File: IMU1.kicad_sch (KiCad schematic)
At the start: 3 parts, among them U2 262-BMI088

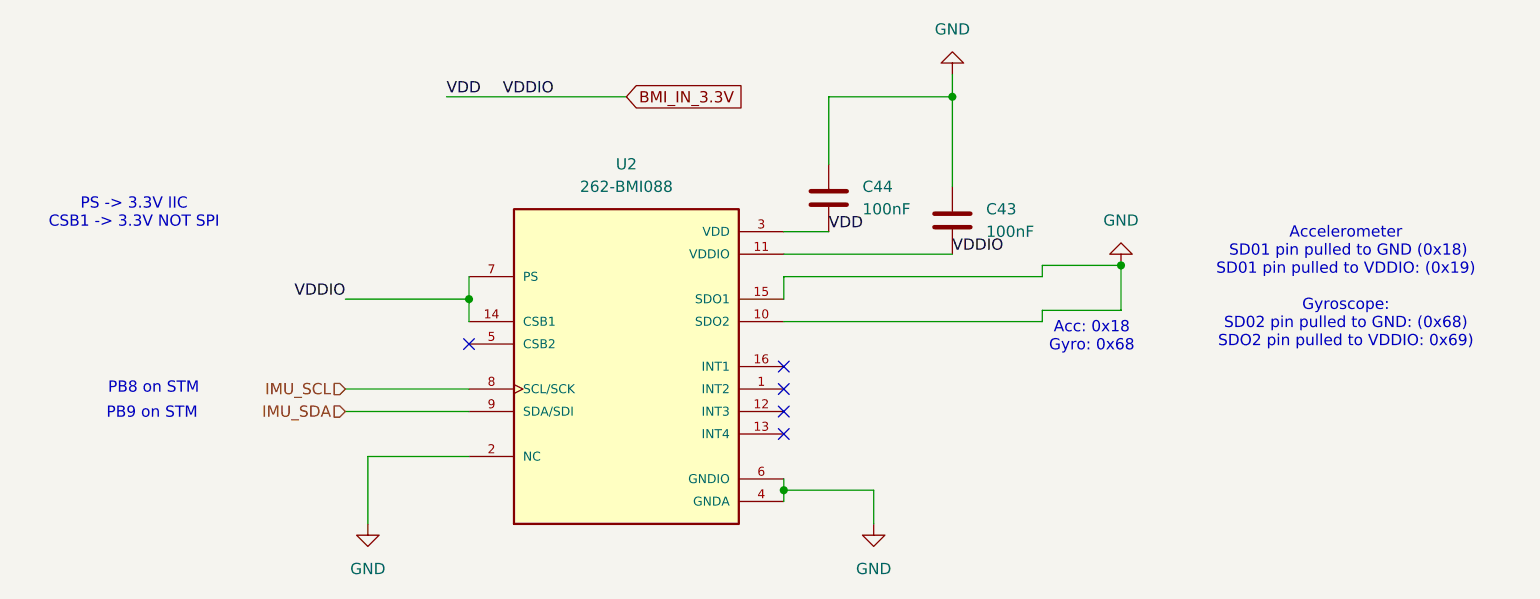
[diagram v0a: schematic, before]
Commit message: multiple chainges on PCB
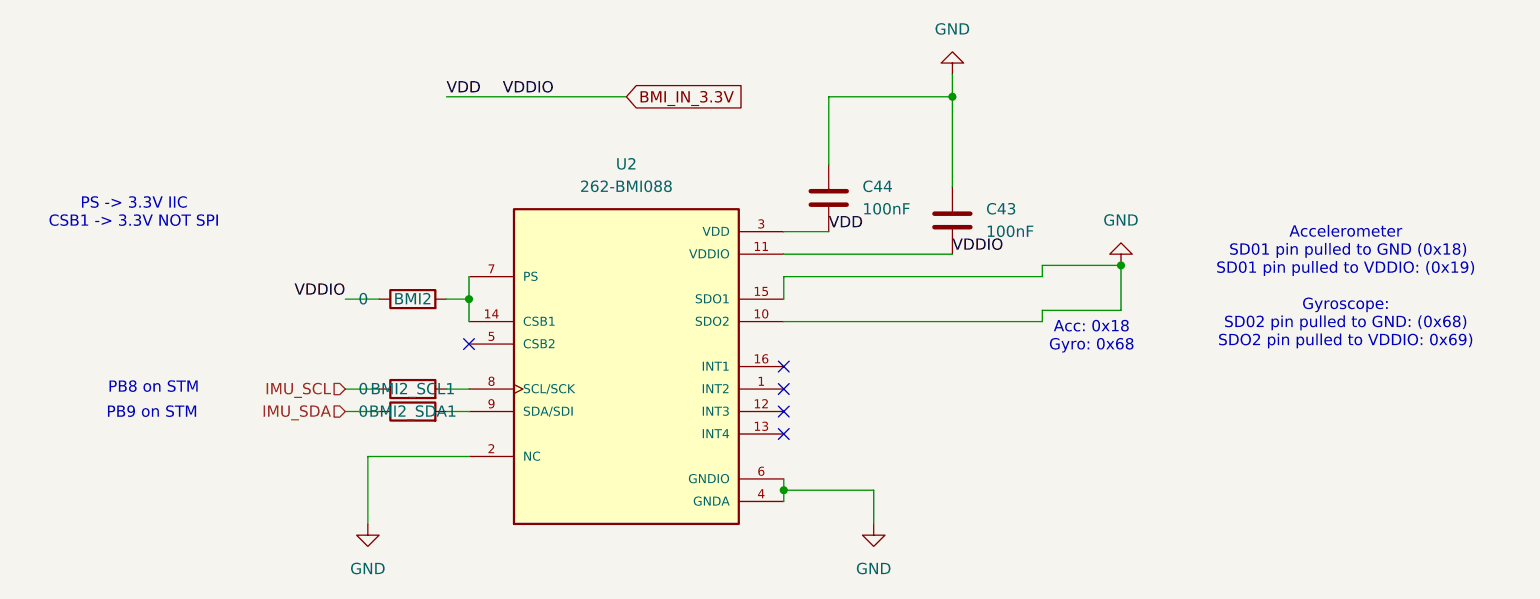
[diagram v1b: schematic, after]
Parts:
- added BMI2, BMI2_SCL1, BMI2_SDA1: 0, Resistor_SMD:R_0603_1608Metric, symbol #dzdb:g_res/R-0-0603
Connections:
- net BMI_IN_3.3V: now also BMI2.1; no longer U2.14 (CSB1), U2.7 (PS)
- net IMU_SCL: now also BMI2_SCL1.1; no longer U2.8 (SCL/SCK)
- net IMU_SDA: now also BMI2_SDA1.1; no longer U2.9 (SDA/SDI)
- new net: BMI2.2, U2.14 (CSB1), U2.7 (PS)
- new net: BMI2_SCL1.2, U2.8 (SCL/SCK)
- new net: BMI2_SDA1.2, U2.9 (SDA/SDI)
